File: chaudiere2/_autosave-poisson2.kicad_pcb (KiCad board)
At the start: 2 copper layers, 100 x 100 mm, 79 parts, among them J1 Conn_02x12_Top_Bottom, J10 Conn_01x02_Female, J11 Screw_Terminal_01x02, J12 Conn_01x02_Female, J13 Screw_Terminal_01x02, J14 Conn_01x02_Female, J15 Screw_Terminal_01x02, J16 Conn_01x02_Female, J17 Screw_Terminal_01x02, J18 Conn_01x02_Female, J19 Conn_01x02_Female, J2 Conn_01x02_Male, J20 Conn_01x02_Female, J21 Conn_01x02_Female, J22 Screw_Terminal_01x02, J23 Screw_Terminal_01x02, J24 Screw_Terminal_01x02, J25 Conn_01x02_Female, J26 Conn_01x02_Female, J27 Conn_01x02_Female, J28 Conn_01x02_Female, J29 Conn_01x02_Female, J3 Conn_01x02_Female, J30 Conn_01x02_Female, J4 Conn_01x02_Female, J5 Conn_01x02_Female, J6 Conn_01x02_Female, J7 Conn_01x02_Female, J8 Conn_02x05_Counter_Clockwise, J9 Conn_02x05_Top_Bottom, Q1 BC548, Q2 BC548, Q3 BC548, Q4 BC548, Q5 BC548, U2 ESP8266EX-NODEMCU-FRED-chaudi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

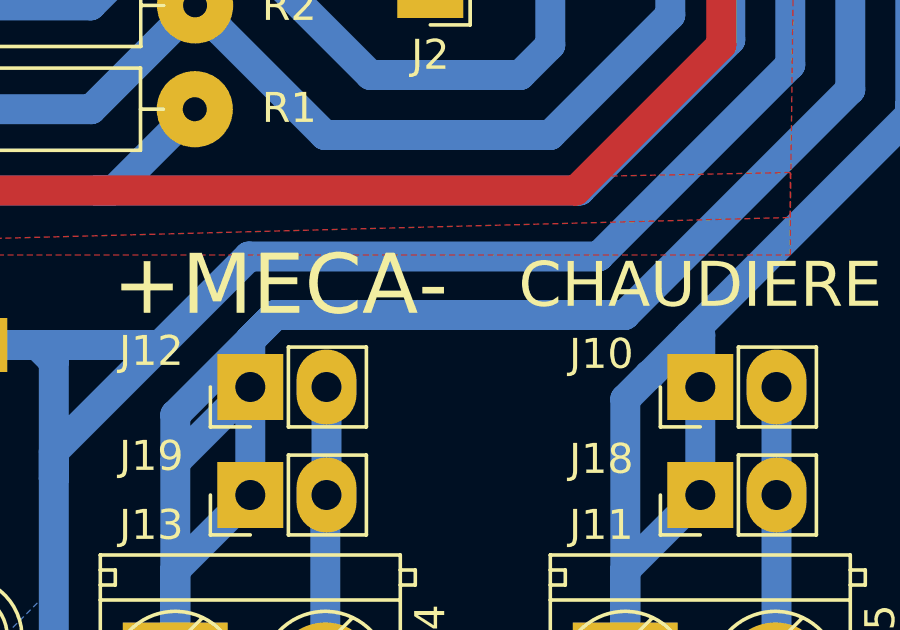
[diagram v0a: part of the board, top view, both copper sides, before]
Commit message: prog aruino
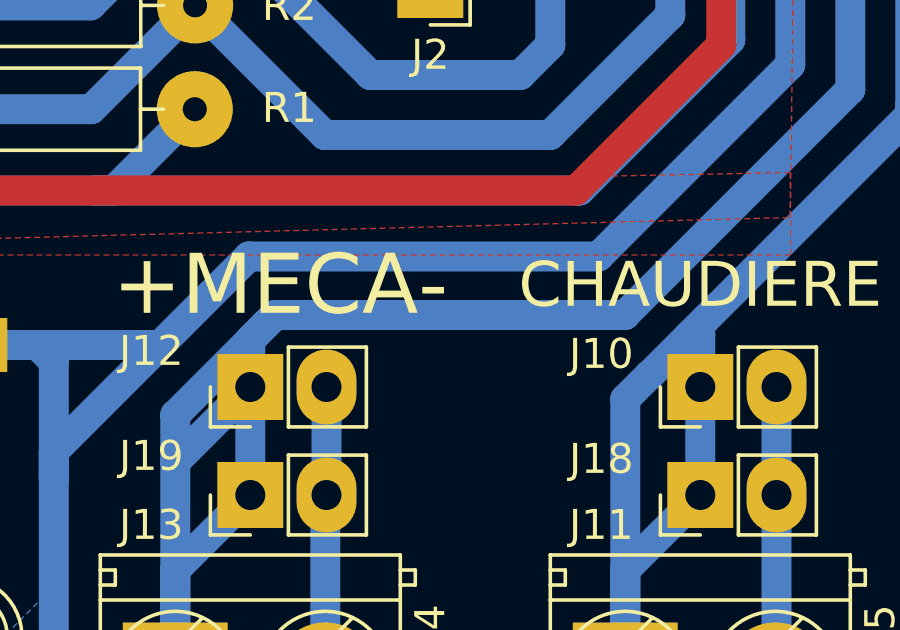
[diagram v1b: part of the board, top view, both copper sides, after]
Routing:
- net Net-(J12-Pad1): track 107.5 -> 110.4 mm
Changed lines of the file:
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@@
     (thickness 1.6)
     (drawings 43)
-    (tracks 728)
+    (tracks 730)
     (zones 0)
     (modules 79)
@@
   (page A4)
   (layers
-    (0 F.Cu signal hide)
+    (0 F.Cu signal)
     (31 B.Cu signal)
     (32 B.Adhes user)
@@
     (47 F.CrtYd user)
     (48 B.Fab user)
-    (49 F.Fab user hide)
+    (49 F.Fab user)
   )
   (setup
@@
   (segment (start 100.00001 118.99999) (end 100.000011 93.981569) (width 1) (layer B.Cu) (net 27))
   (segment (start 84.16 118.68) (end 88.48 123) (width 1) (layer B.Cu) (net 27))
-  (segment (start 98 91.981558) (end 98 76.500787) (width 1) (layer B.Cu) (net 27))
-  (segment (start 98 76.500787) (end 93.449213 71.95) (width 1) (layer B.Cu) (net 27))
   (segment (start 100.000011 93.981569) (end 98 91.981558) (width 1) (layer B.Cu) (net 27))
   (segment (start 93.449213 71.95) (end 92.035 71.95) (width 1) (layer B.Cu) (net 27))
   (segment (start 96 123) (end 100.00001 118.99999) (width 1) (layer B.Cu) (net 27))
   (segment (start 88.48 123) (end 96 123) (width 1) (layer B.Cu) (net 27))
+  (segment (start 98 76.500787) (end 93.449213 71.95) (width 1) (layer B.Cu) (net 27))
+  (segment (start 98 91.981558) (end 98 76.500787) (width 1) (layer B.Cu) (net 27))
   (segment (start 73.32 118) (end 74 118.68) (width 1) (layer B.Cu) (net 28))
   (segment (start 70 118) (end 73.32 118) (width 1) (layer B.Cu) (net 28))
@@
   (segment (start 115.53 89.73) (end 116.626204 89.73) (width 1) (layer B.Cu) (net 43))
   (segment (start 116.626204 89.73) (end 122.000011 84.356193) (width 1) (layer B.Cu) (net 43))
-  (segment (start 86.828409 129.000031) (end 98.485295 129.000031) (width 1) (layer B.Cu) (net 43))
   (segment (start 86 131.4) (end 86 129.82844) (width 1) (layer B.Cu) (net 43))
   (segment (start 98.485295 129.000031) (end 106.000022 121.485304) (width 1) (layer B.Cu) (net 43))
@@
   (segment (start 83.5 132.32844) (end 83.5 133.9) (width 1) (layer B.Cu) (net 43))
   (segment (start 86.828409 129.000031) (end 83.5 132.32844) (width 1) (layer B.Cu) (net 43))
+  (segment (start 95.499969 129.000031) (end 98.471528 129.000031) (width 1) (layer B.Cu) (net 43))
+  (segment (start 95.499969 129.000031) (end 98.485295 129.000031) (width 1) (layer B.Cu) (net 43))
+  (segment (start 86.828409 129.000031) (end 95.499969 129.000031) (width 1) (layer B.Cu) (net 43))
   (segment (start 113.5 137.5) (end 116 135) (width 1) (layer B.Cu) (net 44))
   (segment (start 113.5 141) (end 113.5 137.5) (width 1) (layer B.Cu) (net 44))
